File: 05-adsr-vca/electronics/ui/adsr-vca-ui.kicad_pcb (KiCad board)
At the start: 2 copper layers, 58 x 110 mm, 36 parts, among them J1 Conn_02x03_Odd_Even, J3 Conn_02x03_Odd_Even, J4 Conn_01x02, J5 Conn_01x06, J6 Conn_02x03_Odd_Even, J8 Conn_02x03_Odd_Even, Q1 2N3904, Q2 2N3906

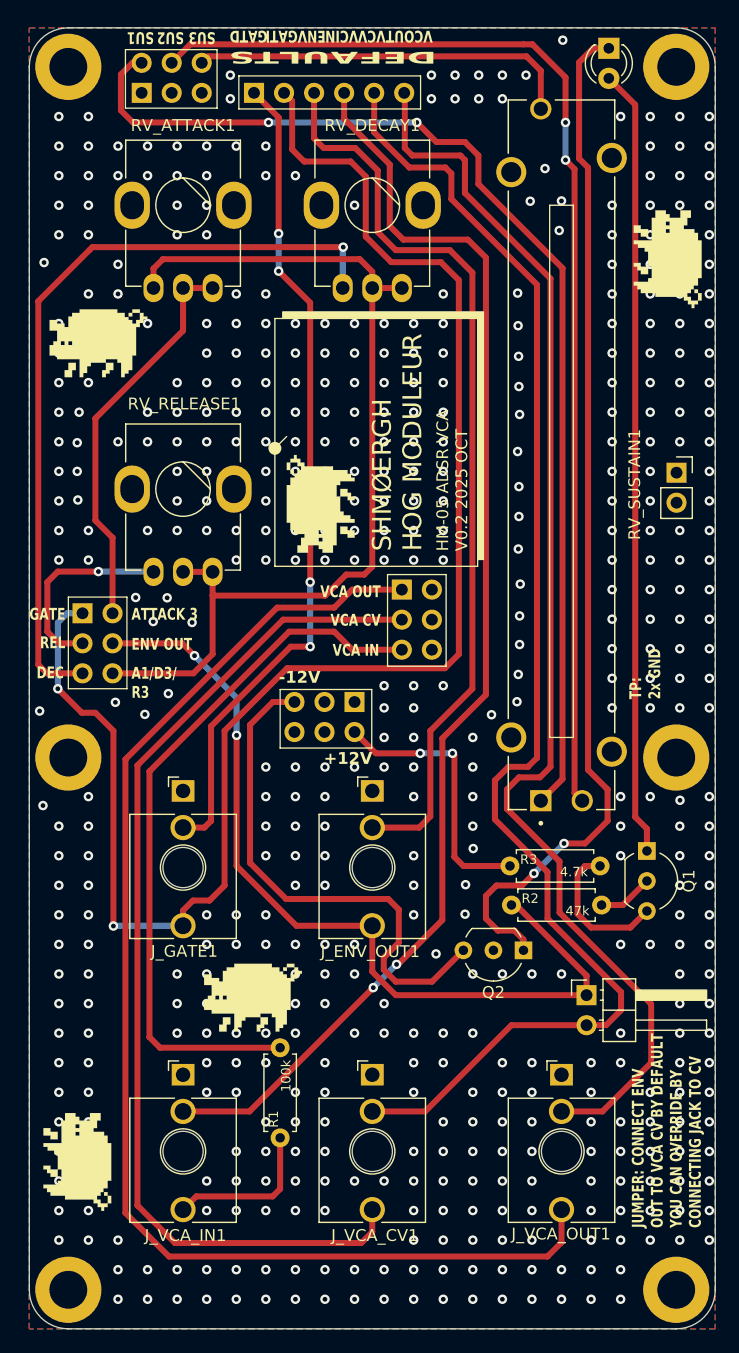
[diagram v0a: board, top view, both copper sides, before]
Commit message: Added VCA amp bias pot
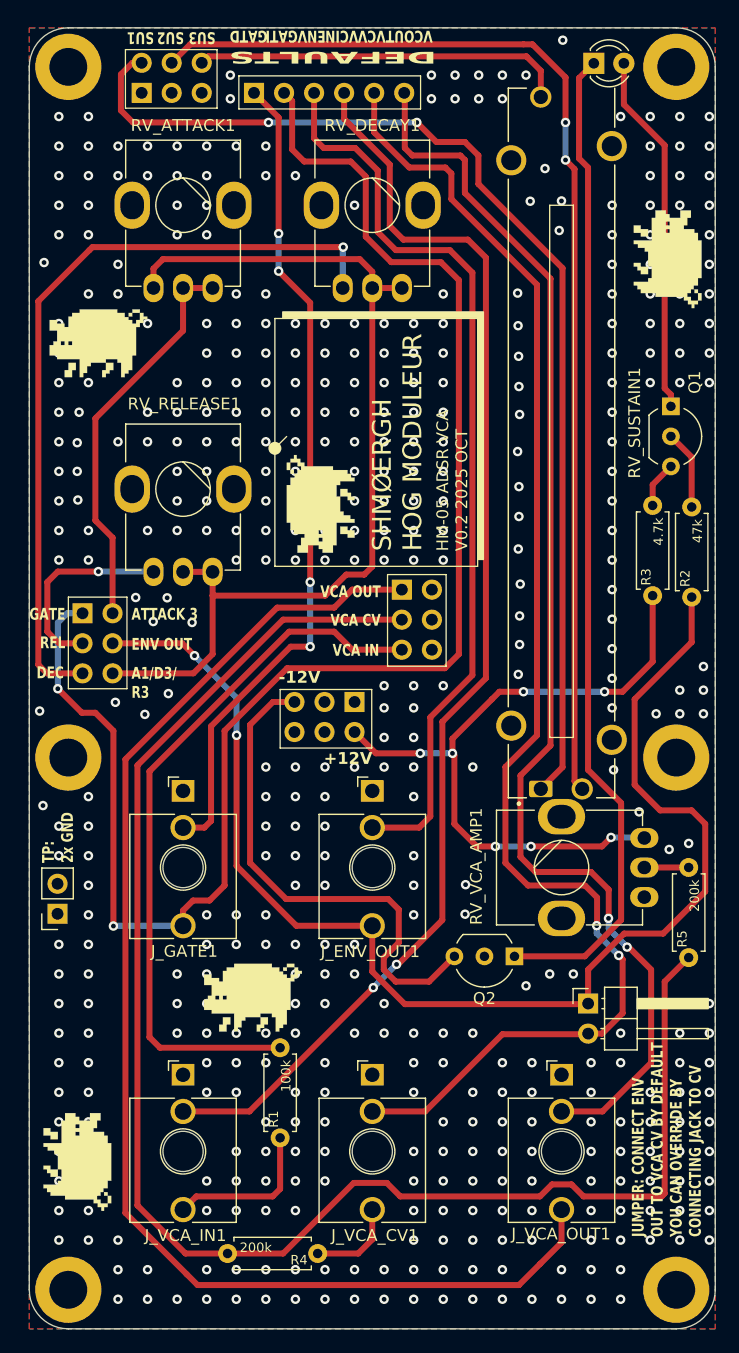
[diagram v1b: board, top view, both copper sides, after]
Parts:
- added R4: 200k, Shmoergh_Custom_Footprints:R_Axial_DIN0207_L6.3mm_D2.5mm_P7.62mm_Horizontal, F.Cu at (148.4, 147.6)
- added R5: 200k, Shmoergh_Custom_Footprints:R_Axial_DIN0207_L6.3mm_D2.5mm_P7.62mm_Horizontal, F.Cu at (179.8, 122.6)
- added RV_VCA_AMP1: 100k, Shmoergh_Custom_Footprints:Potentiometer_Bourns_Single-PTV09A, F.Cu at (169.0, 115.0)
- moved J4 64.3 mm to (126.4, 118.9), turned to 180 degrees
- moved Q1 37.6 mm to (178.2, 76.0)
- moved R2 30.2 mm to (180.0, 92.1), turned to 90 degrees
- moved R3 25.8 mm to (176.7, 92.0), turned to 90 degrees
- moved D1 1.80 mm to (171.7, 47.0), turned to 0 degrees
- moved RV_SUSTAIN1 1.00 mm to (169.0, 79.1)
- moved Q2 0.92 mm to (165.0, 122.5)
- moved JP_DEFAULT_ENV_TO_VCA1 0.72 mm to (171.2, 126.5)
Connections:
- J_VCA_CV1 pad T: VCA_CV -> Net-(J_VCA_CV1-PadT)
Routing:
- net VCA_CV: track 88.1 -> 135.6 mm
- net ENV_OUT: track 73.5 -> 109.9 mm
- net Net-(D1-A): track 66.7 -> 30.7 mm
- net +12V: track 22.9 -> 58.7 mm, vias 2 -> 7
- net Net-(Q1-C): track 12.5 -> 3.94 mm
- net Net-(J_VCA_CV1-PadT): track 0.00 -> 7.63 mm
- net Net-(R5-Pad2): track 0.00 -> 3.76 mm
- net Net-(D1-K): track 87.8 -> 84.7 mm, vias 2 -> 0
- net Net-(Q1-B): track 4.67 -> 6.70 mm
- net VCA_OUT: track 109.3 -> 111.3 mm
- net VCA_CV_DEFAULT: track 116.5 -> 118.0 mm, vias 0 -> 2
- net SUSTAIN_3: track 32.6 -> 31.6 mm
- net SUSTAIN_2: track 96.8 -> 95.8 mm
- net SUSTAIN_1: track 95.3 -> 94.3 mm
- net -12V: track 44.3 -> 43.3 mm
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
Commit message: Reverted VCA to no-bias version
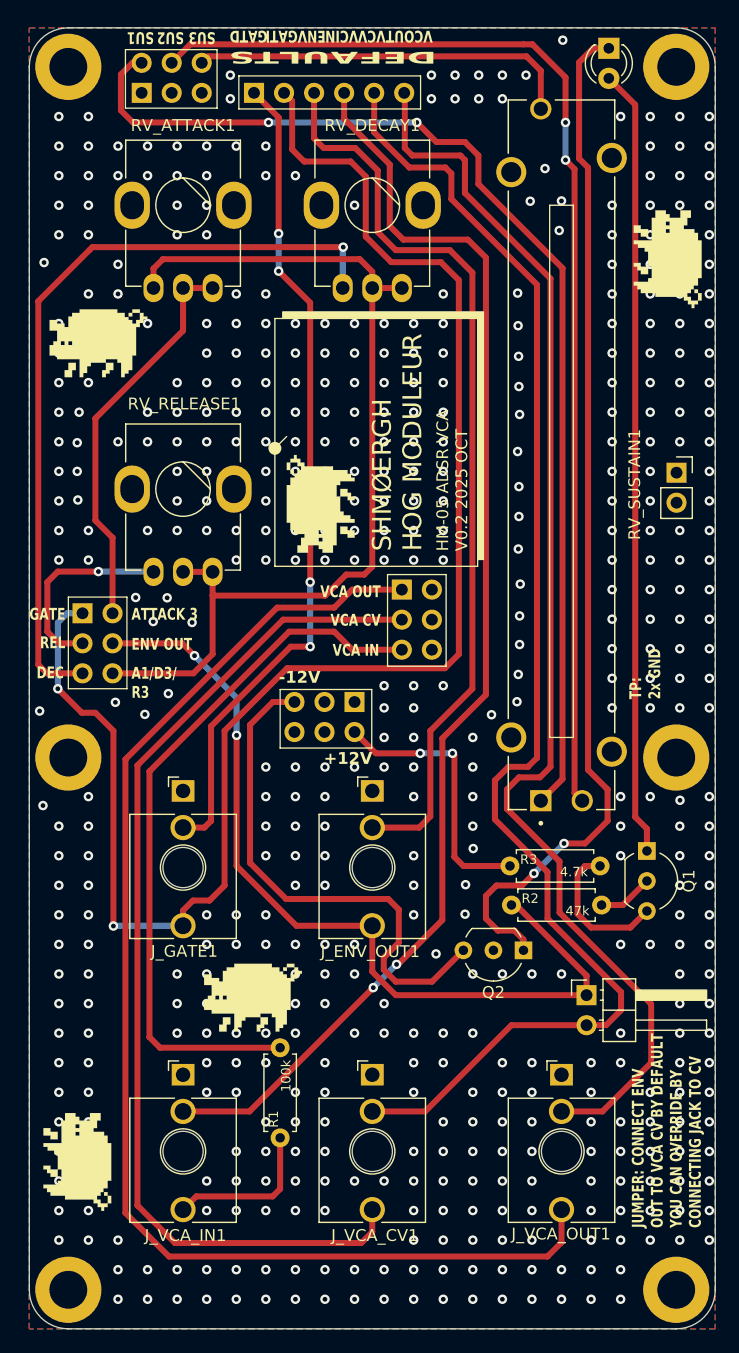
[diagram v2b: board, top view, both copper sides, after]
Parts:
- removed R4, R5: 200k, Shmoergh_Custom_Footprints:R_Axial_DIN0207_L6.3mm_D2.5mm_P7.62mm_Horizontal
- removed RV_VCA_AMP1: 100k, Shmoergh_Custom_Footprints:Potentiometer_Bourns_Single-PTV09A
- moved J4 64.3 mm to (178.7, 81.6), turned to 0 degrees
- moved Q1 37.6 mm to (176.2, 113.6)
- moved R2 30.2 mm to (164.8, 118.2), turned to 0 degrees
- moved R3 25.8 mm to (164.6, 114.9), turned to 0 degrees
- moved D1 1.80 mm to (173.0, 45.7), turned to -90 degrees
- moved RV_SUSTAIN1 1.00 mm to (169.0, 80.1)
- moved Q2 0.92 mm to (165.8, 122.0)
- moved JP_DEFAULT_ENV_TO_VCA1 0.72 mm to (171.1, 125.8)
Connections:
- J_VCA_CV1 pad T: Net-(J_VCA_CV1-PadT) -> VCA_CV
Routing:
- net VCA_CV: track 135.6 -> 88.1 mm
- net ENV_OUT: track 109.9 -> 73.5 mm
- net Net-(D1-A): track 30.7 -> 66.7 mm
- net +12V: track 58.7 -> 22.9 mm, vias 7 -> 2
- net Net-(Q1-C): track 3.94 -> 12.5 mm
- net Net-(J_VCA_CV1-PadT): track 7.63 -> 0.00 mm
- net Net-(R5-Pad2): track 3.76 -> 0.00 mm
- net Net-(D1-K): track 84.7 -> 87.8 mm, vias 0 -> 2
- net Net-(Q1-B): track 6.70 -> 4.67 mm
- net VCA_OUT: track 111.3 -> 109.3 mm
- net VCA_CV_DEFAULT: track 118.0 -> 116.5 mm, vias 2 -> 0
- net SUSTAIN_3: track 31.6 -> 32.6 mm
- net SUSTAIN_2: track 95.8 -> 96.8 mm
- net SUSTAIN_1: track 94.3 -> 95.3 mm
- net -12V: track 43.3 -> 44.3 mm
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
